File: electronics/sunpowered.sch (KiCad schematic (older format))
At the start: 15 parts

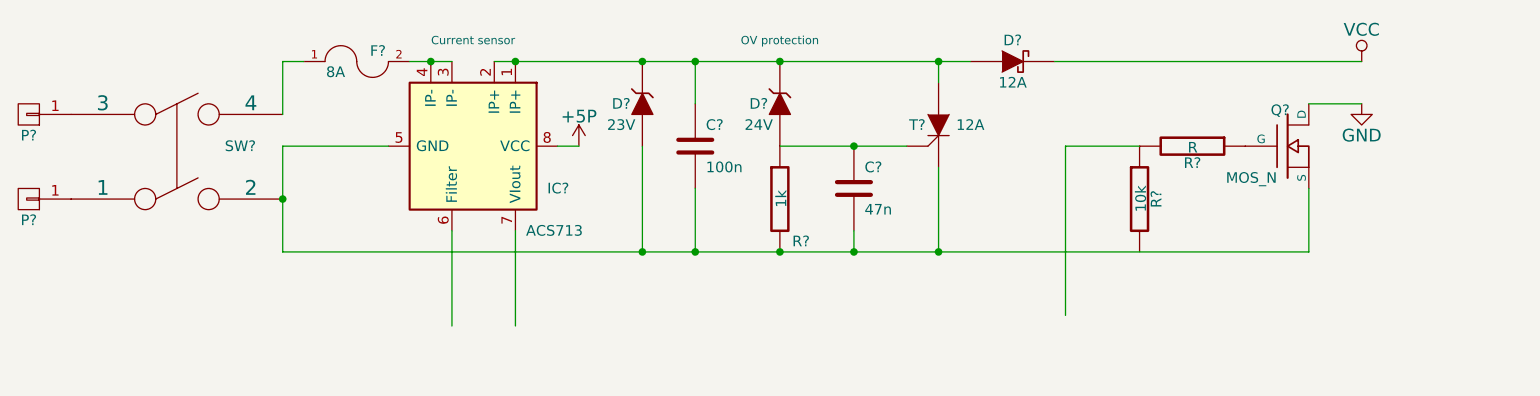
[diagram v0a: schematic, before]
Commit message: minor wires cleanup
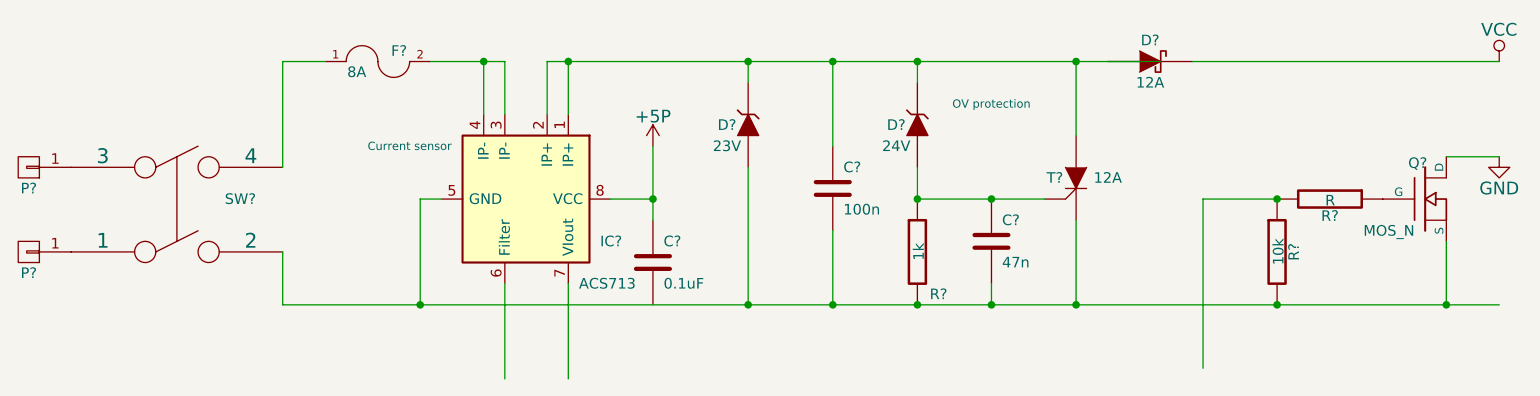
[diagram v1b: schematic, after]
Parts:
- added C?: 0.1uF, symbol C
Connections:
- wire segments 22 -> 45
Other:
- moved on the sheet: C?, D?, F?, IC?, P?, Q?, R?, SW?, T?
